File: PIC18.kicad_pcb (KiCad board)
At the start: 4 copper layers, 76.6 x 75.6 mm, 75 parts, among them J1 Conn_02x20_Odd_Even, J10 Port B, J11 Port C, J12 Port D, J13 Conn_01x03, J14 Conn_01x03, J15 Conn_01x03, J16 Conn_01x03, J2 Conn_01x06, J3 USB_A, J4 Conn_01x03, J5 Conn_01x02, J6 Conn_01x02, J7 USB_OTG, J8 Port A, J9 Port E, U1 PIC18F4620, U2 LM4040DBZ-4.1, U3 FT230XS, Y1 8 MHz

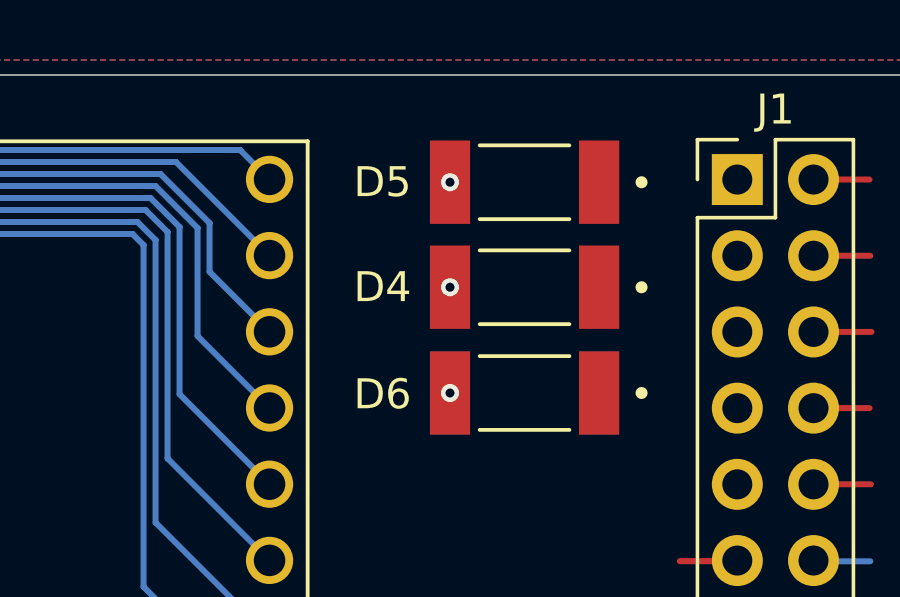
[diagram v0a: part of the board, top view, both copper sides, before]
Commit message: neat
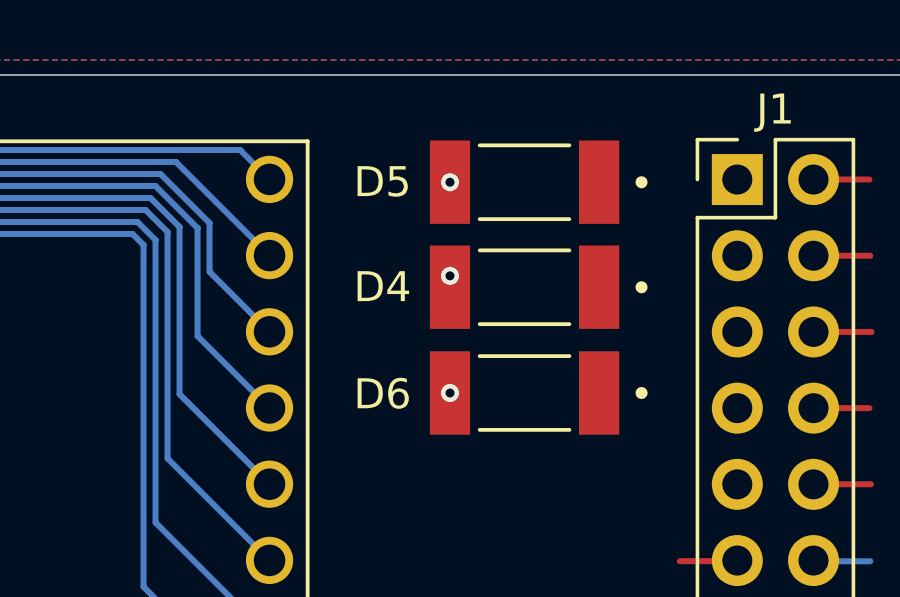
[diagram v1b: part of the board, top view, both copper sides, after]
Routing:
- net /RC1/T1OSI/CCP2(1): track 50.4 -> 53.1 mm
- net /RC2/CCP1/P1A: track 54.3 -> 51.9 mm
- net /OSC2/CLKO/RA6: track 68.3 -> 70.5 mm
- net /RD0/PSP0: track 57.7 -> 55.6 mm
- net /RC0/T1OSO/T13CKI: track 50.3 -> 48.2 mm
- net /OSC1/CLKI/RA7: track 79.7 -> 77.7 mm
- net /RC3/SCK/SCL: track 54.0 -> 56.0 mm
- net /RD1/PSP1: track 57.9 -> 56.4 mm
- net /RA3/AN3/VREF+: track 39.0 -> 37.9 mm
- net /RA4/T0CKI/C1OUT: track 39.6 -> 38.5 mm
- net /RA5/AN4/SS*/HLVDIN/C2OUT: track 40.0 -> 38.9 mm
- net /RE0/RD*/AN5: track 40.4 -> 39.4 mm
- net /RA0/AN0: track 37.3 -> 36.3 mm
- net /RE1/WR*/AN6: track 41.0 -> 40.0 mm
- net /RA1/AN1: track 37.8 -> 36.8 mm
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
